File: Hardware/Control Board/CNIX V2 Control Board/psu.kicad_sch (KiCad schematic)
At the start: 37 parts, among them Q100 MMBTA42, Q101 FDS2734, U100 UCC3803

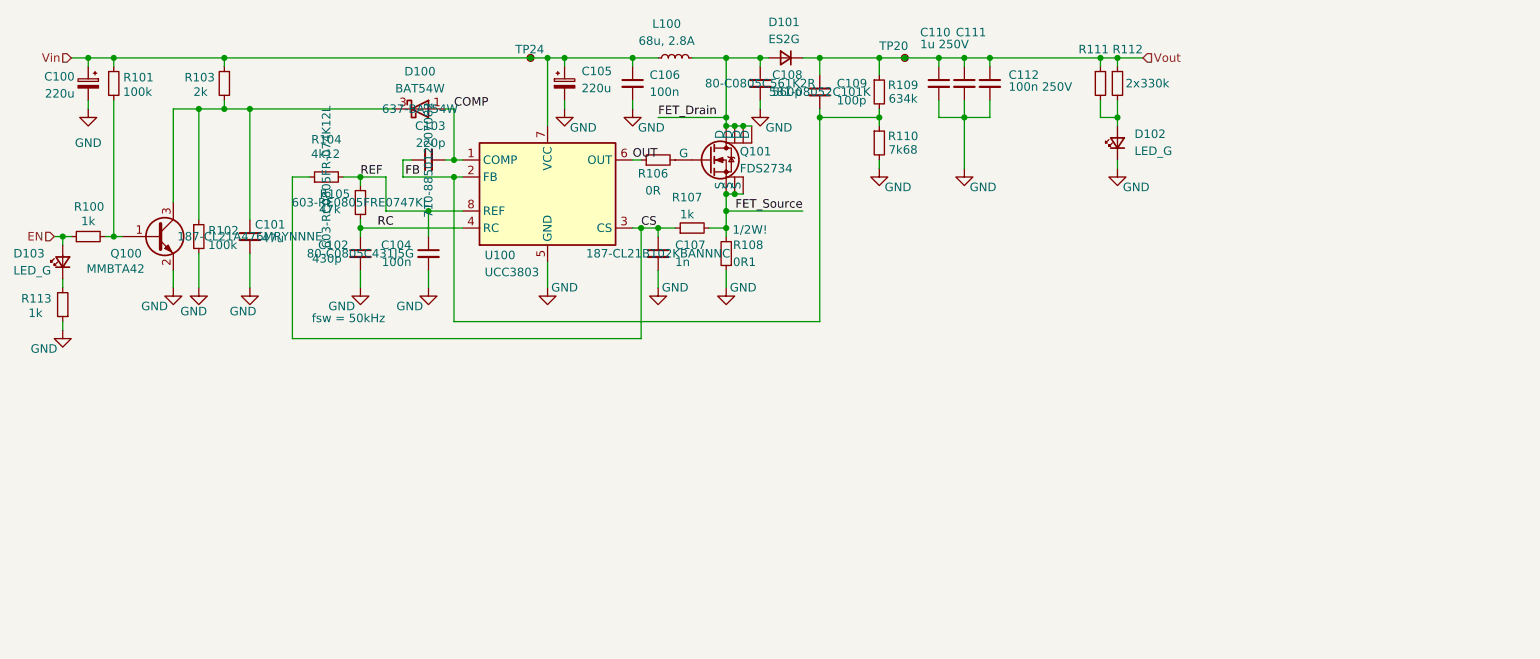
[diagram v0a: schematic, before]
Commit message: fixed schematic
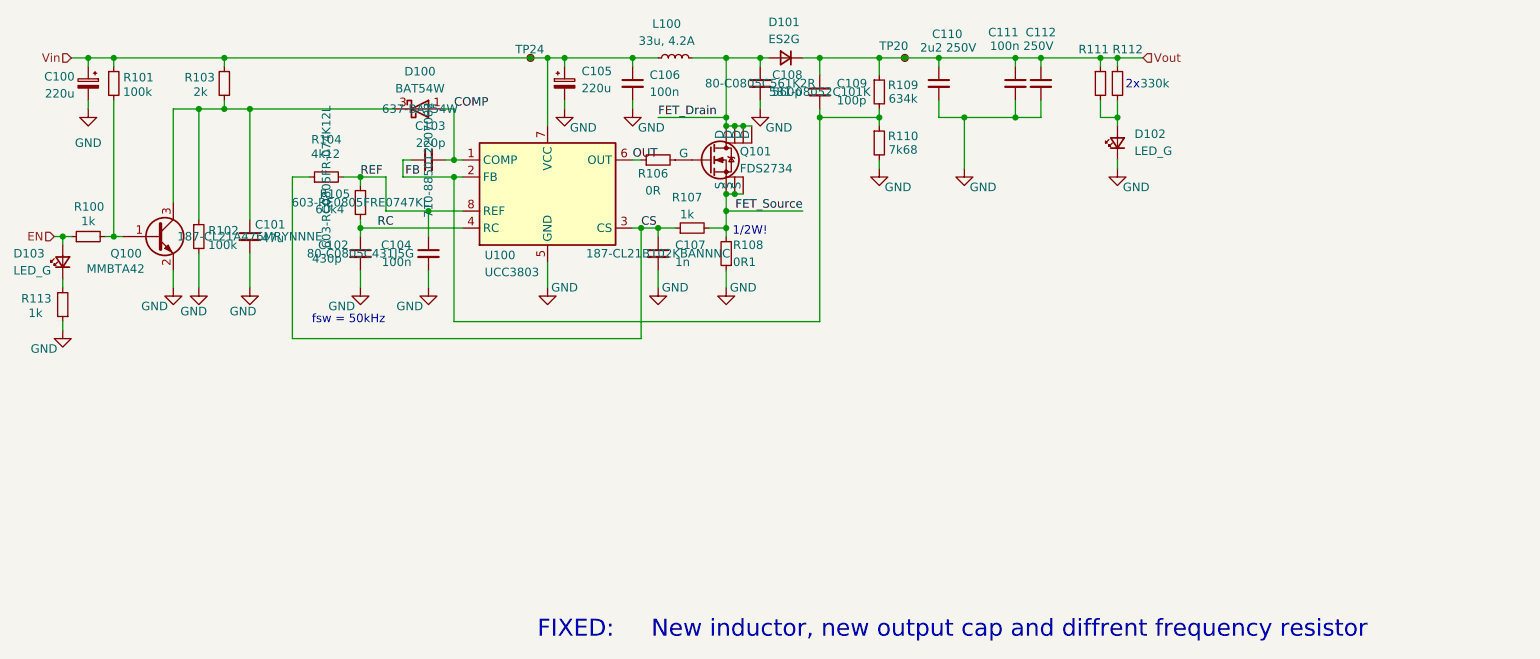
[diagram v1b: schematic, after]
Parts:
- C110: value 1u 250V -> 2u2 250V; footprint Capacitor_SMD:C_0805_2012Metric_Pad1.18x1.45mm_HandSolder -> Capacitor_SMD:C_2220_5750Metric_Pad1.97x5.40mm_HandSolder
- C111: value 1u 250V -> 100nf 250V
- L100: value 68u, 2.8A -> 33u, 4.2A; Mouser Nr. 871-B82477R4683M100 -> 7447709330
- R105: value 47k -> 60k4
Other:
- note added: "FIXED: New inductor, new output cap and diffrent frequency resistor"
- moved on the sheet: C111, C112
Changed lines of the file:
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@@
 		(company "C-Audio")
 	)
+	(text "FIXED: 	New inductor, new output cap and diffrent frequency resistor"
+		(exclude_from_sim no)
+		(at 209.042 156.464 0)
+		(effects
+			(font
+				(size 2.54 2.54)
+			)
+		)
+	)
 	(text "fsw = 50kHz"
 		(exclude_from_sim no)
@@
 	)
 	(junction
+		(at 222.25 71.12)
+		(diameter 0)
+		(color 0 0 0 0)
+	)
+	(junction
 		(at 176.53 81.28)
 		(diameter 0)
@@
 	)
 	(junction
-		(at 210.82 71.12)
+		(at 218.44 71.12)
 		(diameter 0)
 		(color 0 0 0 0)
@@
 	)
 	(junction
-		(at 214.63 71.12)
-		(diameter 0)
-		(color 0 0 0 0)
-	)
-	(junction
 		(at 198.12 80.01)
 		(diameter 0)
@@
 	)
 	(junction
+		(at 218.44 80.01)
+		(diameter 0)
+		(color 0 0 0 0)
+	)
+	(junction
 		(at 233.68 80.01)
 		(diameter 0)
@@
 	(wire
 		(pts
-			(xy 214.63 71.12) (xy 231.14 71.12)
+			(xy 127 88.9) (xy 127 86.36)
 		)
 		(stroke
@@
 	(wire
 		(pts
-			(xy 127 88.9) (xy 127 86.36)
+			(xy 148.59 101.6) (xy 148.59 105.41)
 		)
 		(stroke
@@
 	(wire
 		(pts
-			(xy 148.59 101.6) (xy 148.59 105.41)
+			(xy 218.44 71.12) (xy 222.25 71.12)
 		)
 		(stroke
@@
 	(wire
 		(pts
-			(xy 207.01 71.12) (xy 210.82 71.12)
+			(xy 207.01 71.12) (xy 218.44 71.12)
 		)
 		(stroke
@@
 	(wire
 		(pts
-			(xy 210.82 71.12) (xy 210.82 72.39)
+			(xy 218.44 71.12) (xy 218.44 72.39)
 		)
 		(stroke
@@
 	(wire
 		(pts
-			(xy 214.63 71.12) (xy 214.63 72.39)
+			(xy 222.25 71.12) (xy 222.25 72.39)
 		)
 		(stroke
@@
 	(wire
 		(pts
+			(xy 222.25 71.12) (xy 231.14 71.12)
+		)
+		(stroke
+			(width 0)
+			(type default)
+		)
+	)
+	(wire
+		(pts
 			(xy 120.65 102.87) (xy 120.65 105.41)
 		)
@@
 	(wire
 		(pts
+			(xy 218.44 80.01) (xy 210.82 80.01)
+		)
+		(stroke
+			(width 0)
+			(type default)
+		)
+	)
+	(wire
+		(pts
 			(xy 198.12 71.12) (xy 198.12 73.66)
 		)
@@
 	(wire
 		(pts
-			(xy 214.63 77.47) (xy 214.63 80.01)
+			(xy 222.25 77.47) (xy 222.25 80.01)
 		)
 		(stroke
@@
 	(wire
 		(pts
-			(xy 214.63 80.01) (xy 210.82 80.01)
+			(xy 222.25 80.01) (xy 218.44 80.01)
 		)
 		(stroke
@@
 	(wire
 		(pts
-			(xy 210.82 71.12) (xy 214.63 71.12)
-		)
-		(stroke
-			(width 0)
-			(type default)
-		)
-	)
-	(wire
-		(pts
 			(xy 175.26 71.12) (xy 180.34 71.12)
 		)
@@
 	(wire
 		(pts
-			(xy 210.82 77.47) (xy 210.82 80.01)
+			(xy 218.44 77.47) (xy 218.44 80.01)
 		)
 		(stroke
@@
 	(symbol
 		(lib_id "Device:C_Small")
-		(at 210.82 74.93 0)
+		(at 218.44 74.93 0)
 		(unit 1)
 		(exclude_from_sim no)
@@
 		(dnp no)
 		(property "Reference" "C111"
-			(at 209.55 67.31 0)
+			(at 214.376 67.31 0)
 			(effects
 				(font
@@
 			)
 		)
-		(property "Value" "1u 250V"
-			(at 204.216 69.088 0)
+		(property "Value" "100nf 250V"
+			(at 211.836 69.088 0)
 			(effects
 				(font
@@
 				)
 				(justify left)
+				(hide yes)
 			)
 		)
 		(property "Footprint" "Capacitor_SMD:C_0805_2012Metric_Pad1.18x1.45mm_HandSolder"
-			(at 210.82 74.93 0)
+			(at 218.44 74.93 0)
 			(effects
 				(font
@@
 		)
 		(property "Datasheet" "~"
-			(at 210.82 74.93 0)
+			(at 218.44 74.93 0)
 			(effects
 				(font
@@
 		)
 		(property "Description" "Unpolarized capacitor, small symbol"
-			(at 210.82 74.93 0)
+			(at 218.44 74.93 0)
 			(effects
 				(font
@@
 		)
 		(property "Mouser URL" ""
-			(at 210.82 74.93 0)
+			(at 218.44 74.93 0)
 			(effects
 				(font
@@
 		)
 		(property "Mouser Nr." " 810-CGA4J3X7T2E104MA "
-			(at 210.82 74.93 0)
+			(at 218.44 74.93 0)
 			(effects
 				(font
@@
 		)
 		(property "Mouser-Nr." ""
-			(at 210.82 74.93 0)
+			(at 218.44 74.93 0)
 			(effects
 				(font
@@
 		)
 		(property "Reichelt-Nr." ""
-			(at 210.82 74.93 0)
+			(at 218.44 74.93 0)
 			(effects
 				(font
@@
 	(symbol
 		(lib_id "Device:C_Small")
-		(at 214.63 74.93 0)
+		(at 222.25 74.93 0)
 		(unit 1)
 		(exclude_from_sim no)
@@
 		(dnp no)
 		(property "Reference" "C112"
-			(at 217.424 73.66 0)
+			(at 219.964 67.31 0)
 			(effects
 				(font
@@
 		)
 		(property "Value" "100n 250V"
-			(at 217.424 75.438 0)
+			(at 214.63 69.342 0)
 			(effects
 				(font
@@
 		)
 		(property "Footprint" "Capacitor_SMD:C_0805_2012Metric_Pad1.18x1.45mm_HandSolder"
-			(at 214.63 74.93 0)
+			(at 222.25 74.93 0)
 			(effects
 				(font
@@
 		)
 		(property "Datasheet" "~"
-			(at 214.63 74.93 0)
+			(at 222.25 74.93 0)
 			(effects
 				(font
@@
 		)
 		(property "Description" "Unpolarized capacitor, small symbol"
-			(at 214.63 74.93 0)
+			(at 222.25 74.93 0)
 			(effects
 				(font
@@
 		)
 		(property "Mouser URL" ""
-			(at 214.63 74.93 0)
+			(at 222.25 74.93 0)
 			(effects
 				(font
@@
 		)
 		(property "Mouser Nr." " 810-CGA4J3X7T2E104MA "
-			(at 214.63 74.93 0)
+			(at 222.25 74.93 0)
 			(effects
 				(font
@@
 		)
 		(property "Mouser-Nr." ""
-			(at 214.63 74.93 0)
+			(at 222.25 74.93 0)
 			(effects
 				(font
@@
 		)
 		(property "Reichelt-Nr." ""
-			(at 214.63 74.93 0)
+			(at 222.25 74.93 0)
 			(effects
 				(font
@@
 			)
 		)
-		(property "Value" "68u, 2.8A"
+		(property "Value" "33u, 4.2A"
 			(at 166.37 68.58 90)
 			(effects
@@
 			)
 		)
-		(property "Mouser Nr." " 871-B82477R4683M100 "
+		(property "Mouser Nr." "7447709330"
 			(at 167.64 71.12 0)
 			(effects
@@
 		(dnp no)
 		(property "Reference" "C110"
-			(at 204.216 67.31 0)
+			(at 205.994 67.564 0)
 			(effects
 				(font
@@
 			)
 		)
-		(property "Value" "1u 250V"
-			(at 209.55 76.2062 0)
+		(property "Value" "2u2 250V"
+			(at 204.216 69.596 0)
 			(effects
 				(font
@@
 				)
 				(justify left)
-				(hide yes)
 			)
 		)
-		(property "Footprint" "Capacitor_SMD:C_0805_2012Metric_Pad1.18x1.45mm_HandSolder"
+		(property "Footprint" "Capacitor_SMD:C_2220_5750Metric_Pad1.97x5.40mm_HandSolder"
 			(at 207.01 74.93 0)
 			(effects
@@
 			)
 		)
-		(property "Value" "47k"
+		(property "Value" "60k4"
 			(at 116.078 93.726 0)
 			(effects
